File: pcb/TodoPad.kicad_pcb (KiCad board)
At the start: 2 copper layers, 99 x 96.7 mm, 30 parts, among them SW1 SW_Push, SW10 SW_Push, SW11 SW_Push, SW12 SW_Push, SW13 SW_Push, SW14 SW_Push, SW2 SW_Push, SW3 SW_Push, SW4 SW_Push, SW5 SW_Push, SW6 SW_Push, SW7 SW_Push, SW8 SW_Push, SW9 SW_Push, U1 XIAO-RP2040-DIP, U2 SSD1306_128x32_OLED_Display

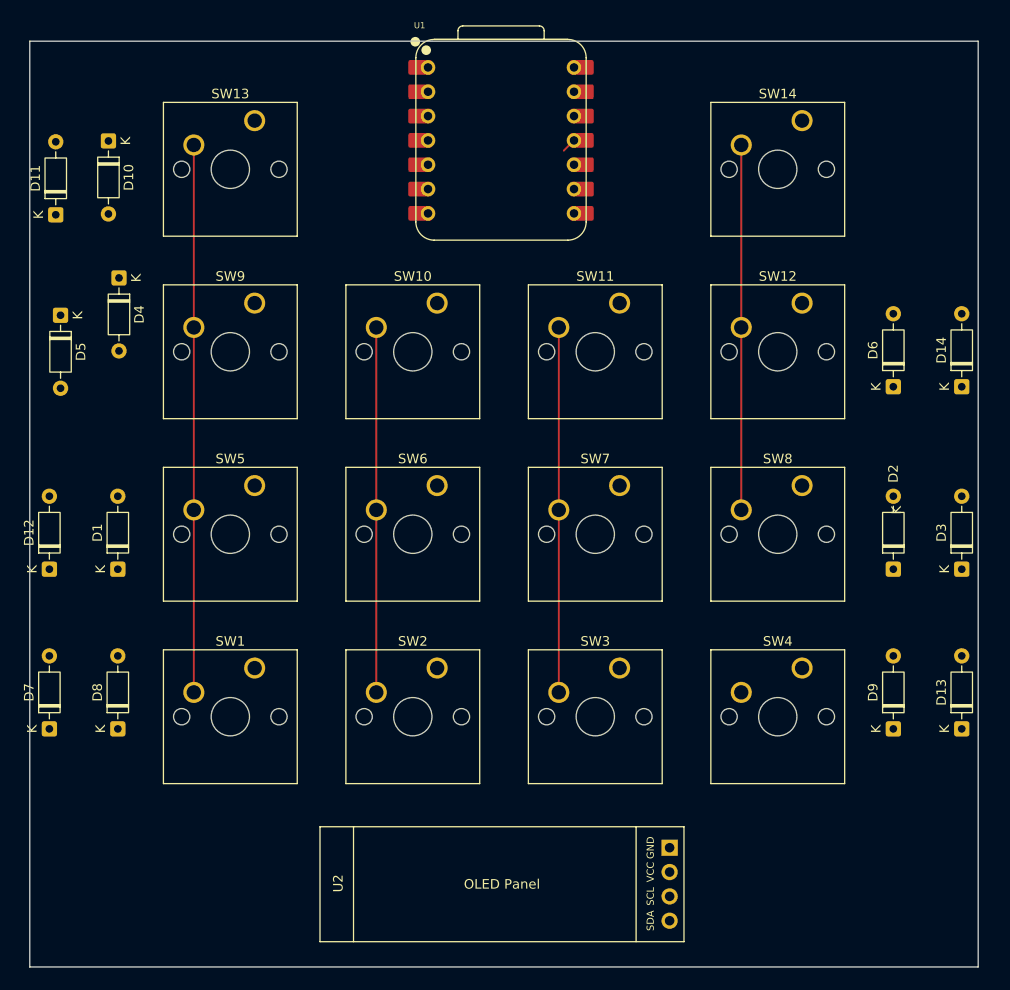
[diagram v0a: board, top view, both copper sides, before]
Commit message: Routing first attempt is complete
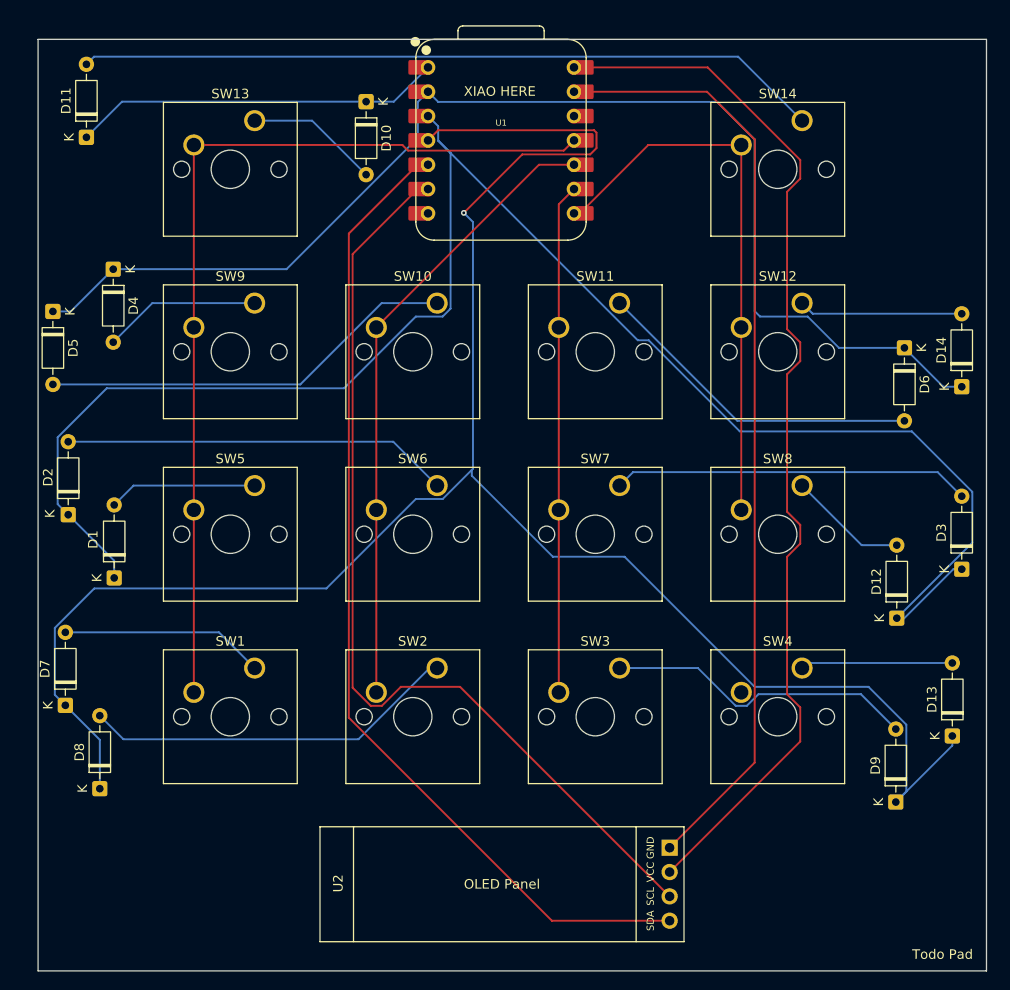
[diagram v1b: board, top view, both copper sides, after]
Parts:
- moved D12 88.6 mm to (180.5, 106.7)
- moved D2 86.3 mm to (94.0, 95.9)
- moved D10 27.2 mm to (125.1, 52.8)
- moved D11 8.70 mm to (95.9, 56.5)
- moved D9 7.65 mm to (180.4, 125.9)
- moved D8 6.52 mm to (97.3, 124.5)
- moved D6 4.22 mm to (181.3, 78.5), turned to -90 degrees
- moved D7 2.97 mm to (93.7, 115.8)
- moved D13 1.23 mm to (186.3, 119.0)
- moved D4 1.09 mm to (98.7, 70.3)
- moved D1 0.99 mm to (98.8, 102.5)
- moved D5 0.89 mm to (92.4, 74.7)
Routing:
- net Row 3: track 0.00 -> 207.4 mm, vias 0 -> 1
- net Row 2: track 0.00 -> 181.6 mm
- net Row 1: track 0.00 -> 129.8 mm
- net +5V: track 0.00 -> 111.0 mm
- net Net-(U1-GPIO6/SDA): track 0.00 -> 104.1 mm
- net Net-(U1-GPIO7/SCL): track 0.00 -> 99.7 mm
- net GND: track 0.00 -> 98.6 mm
- net Net-(D11-A): track 0.00 -> 77.8 mm
- net Net-(D5-A): track 0.00 -> 43.6 mm
- net Net-(D2-A): track 0.00 -> 40.4 mm
- net Net-(D8-A): track 0.00 -> 39.3 mm
- net Col 0: track 58.7 -> 97.5 mm
- net Row 0: track 0.00 -> 38.7 mm
- net Net-(D3-A): track 0.00 -> 37.3 mm
- net Net-(D6-A): track 0.00 -> 34.8 mm
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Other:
- board size 99 x 96.7 mm -> 99 x 97.2 mm
- board text added: "Todo Pad"
- board text added: "XIAO HERE"
